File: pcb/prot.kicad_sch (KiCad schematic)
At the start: 17 parts, among them J1 Conn_01x05_Pin

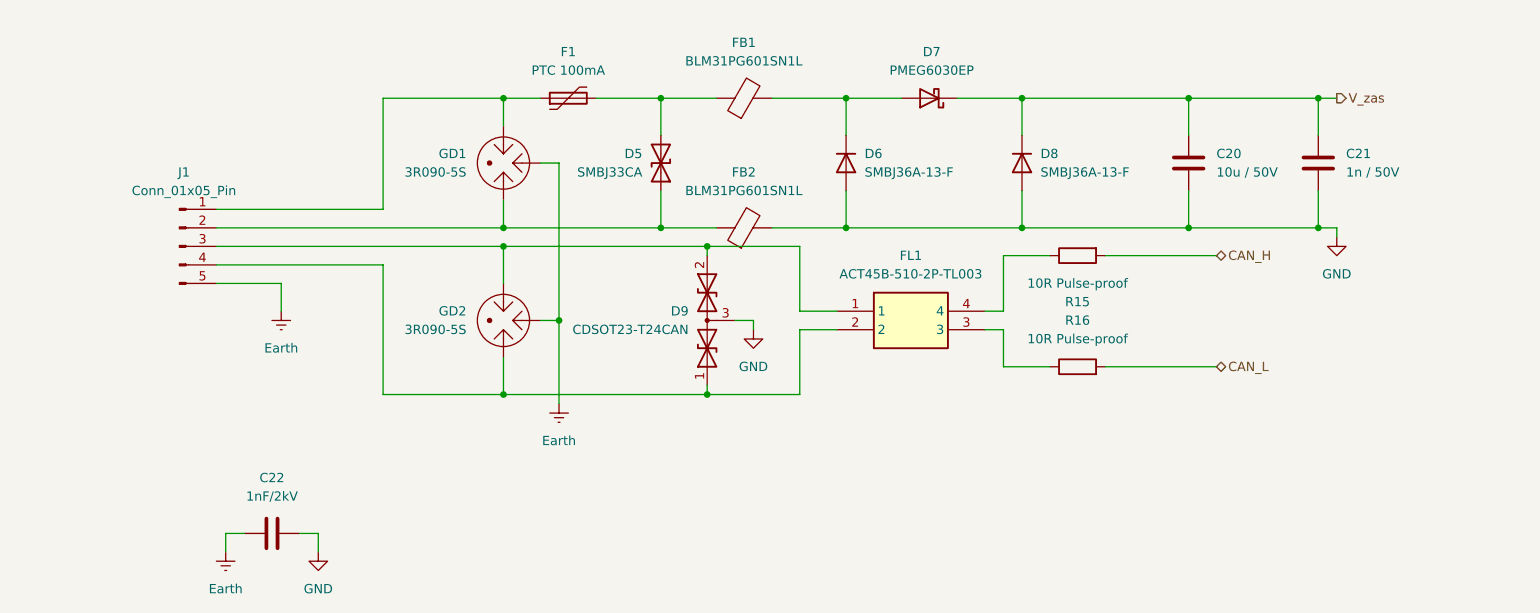
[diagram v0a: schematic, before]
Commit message: Schematic finished, first routing
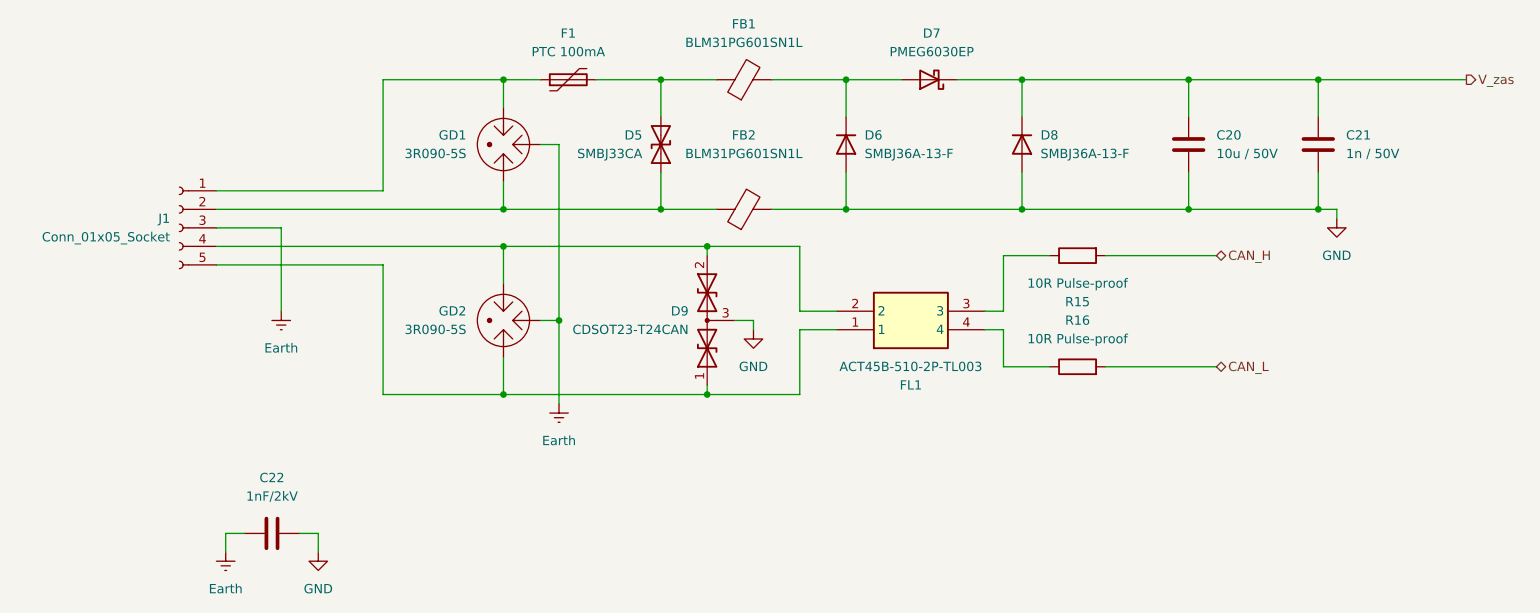
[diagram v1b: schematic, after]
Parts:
- removed J1: Conn_01x05_Pin, Connector_PinHeader_2.00mm:PinHeader_1x05_P2.00mm_Vertical, symbol Connector:Conn_01x05_Pin
- added J1: Conn_01x05_Socket, Connector_PinHeader_2.54mm:PinHeader_1x05_P2.54mm_Vertical, symbol Connector:Conn_01x05_Socket
- D5: footprint (none) -> Diode_SMD:D_SMB
- FL1: footprint ACT45B1012PTL003 -> SamacSys_Parts:ACT45B1012PTL003
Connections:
- net Earth: now also J1.3 (Pin_3)
- net at F1.1, GD1.1: now also J1.1 (Pin_1)
- net at D5.1 (A1), FB2.1, GD1.3: now also J1.2 (Pin_2)
- net at D9.2 (A2), GD2.1: now also FL1.2, J1.4 (Pin_4); no longer FL1.1
- net at D9.1 (A1), GD2.3: now also FL1.1, J1.5 (Pin_5); no longer FL1.2
- net at FL1.3: now also R15.1; no longer R16.1
- net at FL1.4: now also R16.1; no longer R15.1
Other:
- moved on the sheet: C20, C21, D5, D6, D7, D8, F1, FB1, FB2, GD1

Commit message: Cleaning
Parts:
- D5: Manufacturer_Part_Number (none) -> SMBJ33CA
- D6, D8: Manufacturer_Part_Number (none) -> SMBJ36A-13-F
- D7: Manufacturer_Part_Number (none) -> PMEG6030EP
- D9: Manufacturer_Part_Number (none) -> CDSOT23-T24CAN
- F1: Manufacturer_Part_Number (none) -> SN010-60
- FB1, FB2: Manufacturer_Part_Number (none) -> BLM31PG601SN1L
- GD1, GD2: Manufacturer_Part_Number (none) -> Leiditech 3R090-5S
- J1: now left out of the parts list
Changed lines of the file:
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@@
+			)
+		)
+		(property "Manufacturer_Part_Number" "PMEG6030EP"
+			(at 161.29 71.12 0)
+			(hide yes)
+			(show_name no)
+			(do_not_autoplace no)
+			(effects
+				(font
+					(size 1.27 1.27)
+				)
 			)
 		)
@@
 			)
 		)
+		(property "Manufacturer_Part_Number" "SMBJ33CA"
+			(at 124.46 80.01 90)
+			(hide yes)
+			(show_name no)
+			(do_not_autoplace no)
+			(effects
+				(font
+					(size 1.27 1.27)
+				)
+			)
+		)
 		(pin "2"
 		)
@@
 		(body_style 1)
 		(exclude_from_sim no)
-		(in_bom yes)
+		(in_bom no)
 		(on_board yes)
 		(in_pos_files yes)
@@
 			)
 		)
+		(property "Manufacturer_Part_Number" "SN010-60"
+			(at 111.76 71.12 90)
+			(hide yes)
+			(show_name no)
+			(do_not_autoplace no)
+			(effects
+				(font
+					(size 1.27 1.27)
+				)
+			)
+		)
 		(pin "1"
 		)
@@
 			)
 		)
+		(property "Manufacturer_Part_Number" "SMBJ36A-13-F"
+			(at 173.99 80.01 90)
+			(hide yes)
+			(show_name no)
+			(do_not_autoplace no)
+			(effects
+				(font
+					(size 1.27 1.27)
+				)
+			)
+		)
 		(pin "1"
 		)
@@
 			)
 		)
+		(property "Manufacturer_Part_Number" "BLM31PG601SN1L"
+			(at 135.89 71.12 90)
+			(hide yes)
+			(show_name no)
+			(do_not_autoplace no)
+			(effects
+				(font
+					(size 1.27 1.27)
+				)
+			)
+		)
 		(pin "2"
 		)
@@
 			)
 		)
+		(property "Manufacturer_Part_Number" "SMBJ36A-13-F"
+			(at 149.86 80.01 90)
+			(hide yes)
+			(show_name no)
+			(do_not_autoplace no)
+			(effects
+				(font
+					(size 1.27 1.27)
+				)
+			)
+		)
 		(pin "1"
 		)
@@
 			)
 		)
+		(property "Manufacturer_Part_Number" "Leiditech 3R090-5S"
+			(at 102.87 104.14 0)
+			(hide yes)
+			(show_name no)
+			(do_not_autoplace no)
+			(effects
+				(font
+					(size 1.27 1.27)
+				)
+			)
+		)
 		(pin "2"
 		)
@@
 			)
 		)
+		(property "Manufacturer_Part_Number" "Leiditech 3R090-5S"
+			(at 102.87 80.01 0)
+			(hide yes)
+			(show_name no)
+			(do_not_autoplace no)
+			(effects
+				(font
+					(size 1.27 1.27)
+				)
+			)
+		)
 		(pin "2"
 		)
@@
 		(property "Description" "BLM31PG601SN1L"
 			(at 135.89 88.9 0)
+			(hide yes)
+			(show_name no)
+			(do_not_autoplace no)
+			(effects
+				(font
+					(size 1.27 1.27)
+				)
+			)
+		)
+		(property "Manufacturer_Part_Number" "BLM31PG601SN1L"
+			(at 135.89 88.9 90)
 			(hide yes)
 			(show_name no)
@@
 			(hide yes)
 			(show_name no)
+			(do_not_autoplace no)
+			(effects
+				(font
+					(size 1.27 1.27)
+				)
+			)
+		)
+		(property "Manufacturer_Part_Number" "CDSOT23-T24CAN"
+			(at 130.81 104.14 90)
+			(hide yes)
+			(show_name no)
